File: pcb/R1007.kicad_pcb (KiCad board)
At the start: 2 copper layers, 45 x 33.3 mm, 1 part, among them J1 PCIEx1Edge

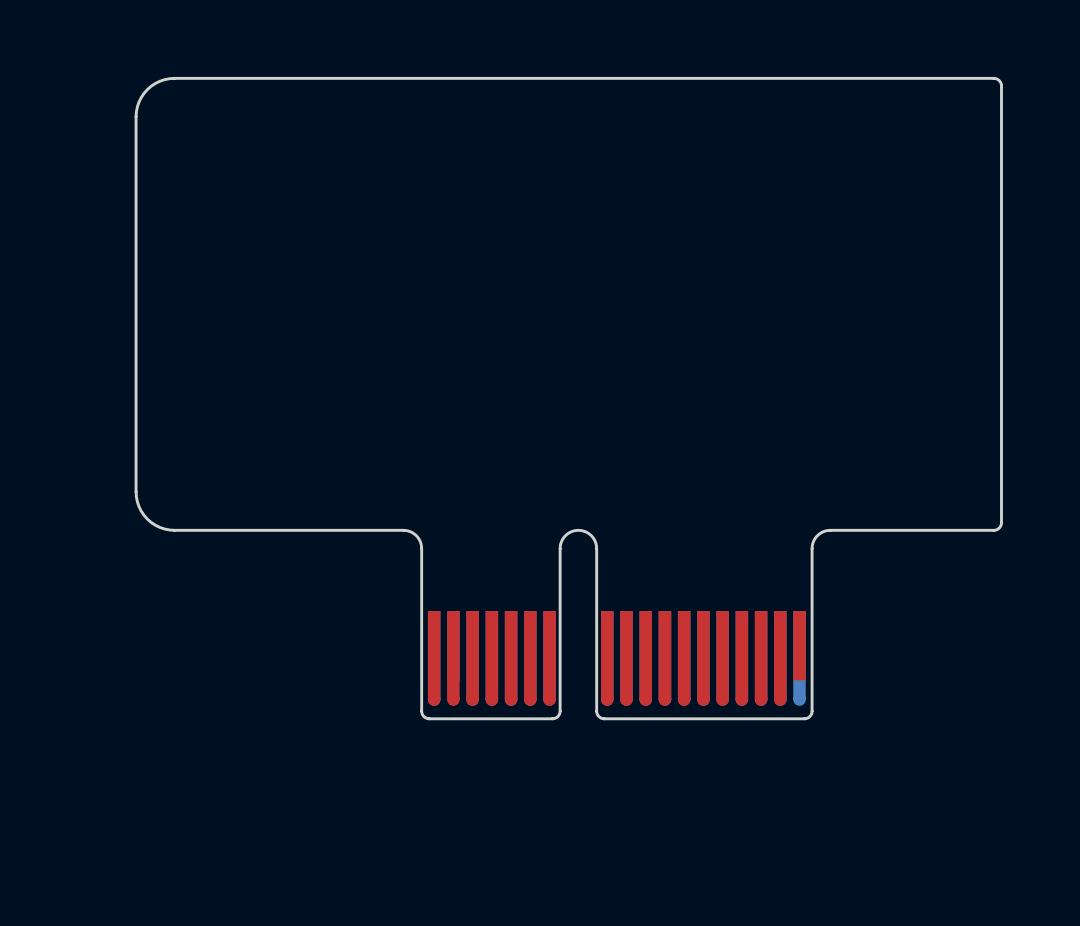
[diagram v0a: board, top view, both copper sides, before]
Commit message: wip, need to add 74 buffers and LEDs
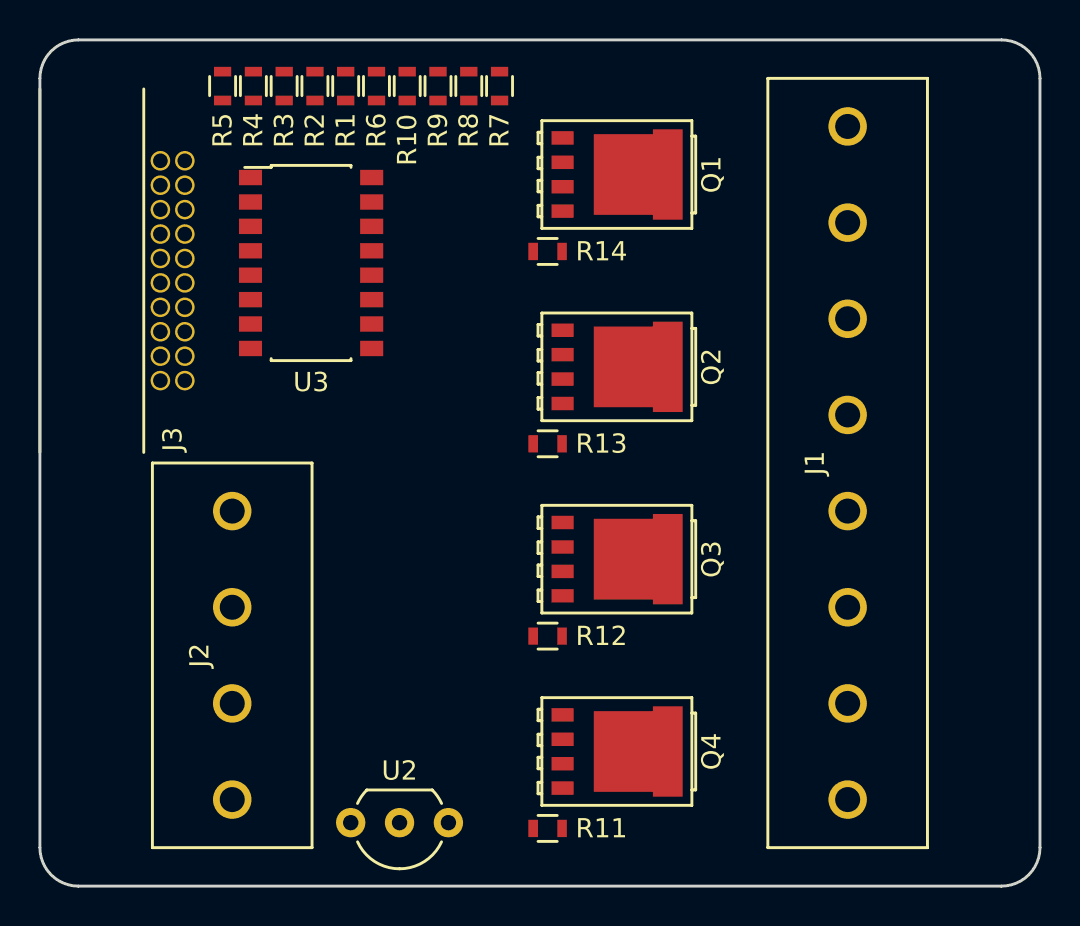
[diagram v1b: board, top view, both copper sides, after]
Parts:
- added J2: CONN500P-01X04, Main:CONN500P-01X04, F.Cu at (130.0, 100.0)
- added J3: CONN_R1000A_EXTENSION, Main:CONN127P-02X10, F.Cu at (126.9, 80.0)
- added Q1: PSMN1R2-30YLC, Main:SOT127P500X110-5, F.Cu at (150.0, 75.0)
- added Q2: PSMN1R2-30YLC, Main:SOT127P500X110-5, F.Cu at (150.0, 85.0)
- added Q3: PSMN1R2-30YLC, Main:SOT127P500X110-5, F.Cu at (150.0, 95.0)
- added Q4: PSMN1R2-30YLC, Main:SOT127P500X110-5, F.Cu at (150.0, 105.0)
- added R1: 10k, Resistors_SMD:R_0603, F.Cu at (135.9, 70.4)
- added R10: 10k, Resistors_SMD:R_0603, F.Cu at (139.1, 70.4)
- added R11: 10k, Resistors_SMD:R_0603, F.Cu at (146.4, 109.0)
- added R12: 10k, Resistors_SMD:R_0603, F.Cu at (146.4, 99.0)
- added R13: 10k, Resistors_SMD:R_0603, F.Cu at (146.4, 89.0)
- added R14: 10k, Resistors_SMD:R_0603, F.Cu at (146.4, 79.0)
- added R2: 10k, Resistors_SMD:R_0603, F.Cu at (134.3, 70.4)
- added R3: 10k, Resistors_SMD:R_0603, F.Cu at (132.7, 70.4)
- added R4: 10k, Resistors_SMD:R_0603, F.Cu at (131.1, 70.4)
- added R5: 10k, Resistors_SMD:R_0603, F.Cu at (129.5, 70.4)
- added R6: 10k, Resistors_SMD:R_0603, F.Cu at (137.5, 70.4)
- added R7: 10k, Resistors_SMD:R_0603, F.Cu at (143.9, 70.4)
- added R8: 10k, Resistors_SMD:R_0603, F.Cu at (142.3, 70.4)
- added R9: 10k, Resistors_SMD:R_0603, F.Cu at (140.7, 70.4)
- added U2: AS78L05ZTR-E1, Main:TO92_AMMO, F.Cu at (138.7, 108.7)
- added U3: TLP293-4, Main:SOIC127P1030X455X210-16, F.Cu at (134.1, 79.6)
- J1: value PCIEx1Edge -> CONN500P-01X08; footprint Main:PCIEXPRESS-X1 -> Main:CONN500P-01X08; moved to F.Cu
- moved J1 15.6 mm to (162.0, 90.0), turned to 90 degrees
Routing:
- net Net-(J1-PadB9): track 2.30 -> 0.00 mm
- net Net-(J1-PadB8): track 2.30 -> 0.00 mm
- net Net-(J1-PadB7): track 2.30 -> 0.00 mm
- net Net-(J1-PadB6): track 2.30 -> 0.00 mm
- net Net-(J1-PadB5): track 2.30 -> 0.00 mm
- net Net-(J1-PadB4): track 2.30 -> 0.00 mm
- net Net-(J1-PadB3): track 2.30 -> 0.00 mm
- net Net-(J1-PadB2): track 2.30 -> 0.00 mm
- net Net-(J1-PadB18): track 2.30 -> 0.00 mm
- net Net-(J1-PadB16): track 2.30 -> 0.00 mm
- net Net-(J1-PadB15): track 2.30 -> 0.00 mm
- net Net-(J1-PadB14): track 2.30 -> 0.00 mm
- net Net-(J1-PadB13): track 2.30 -> 0.00 mm
- net Net-(J1-PadB12): track 2.30 -> 0.00 mm
- net Net-(J1-PadB11): track 2.30 -> 0.00 mm
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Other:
- board size 45 x 33.3 mm -> 52 x 44 mm
- copper layers 2 -> 4
